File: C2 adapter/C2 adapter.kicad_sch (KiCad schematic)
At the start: 13 parts, among them J1 Conn_01x08_Pin, J2 Conn_02x05_Counter_Clockwise, J3 Conn_01x08_Socket, Q1 Q_NPN_BCE, U1 BAV23CLT1G

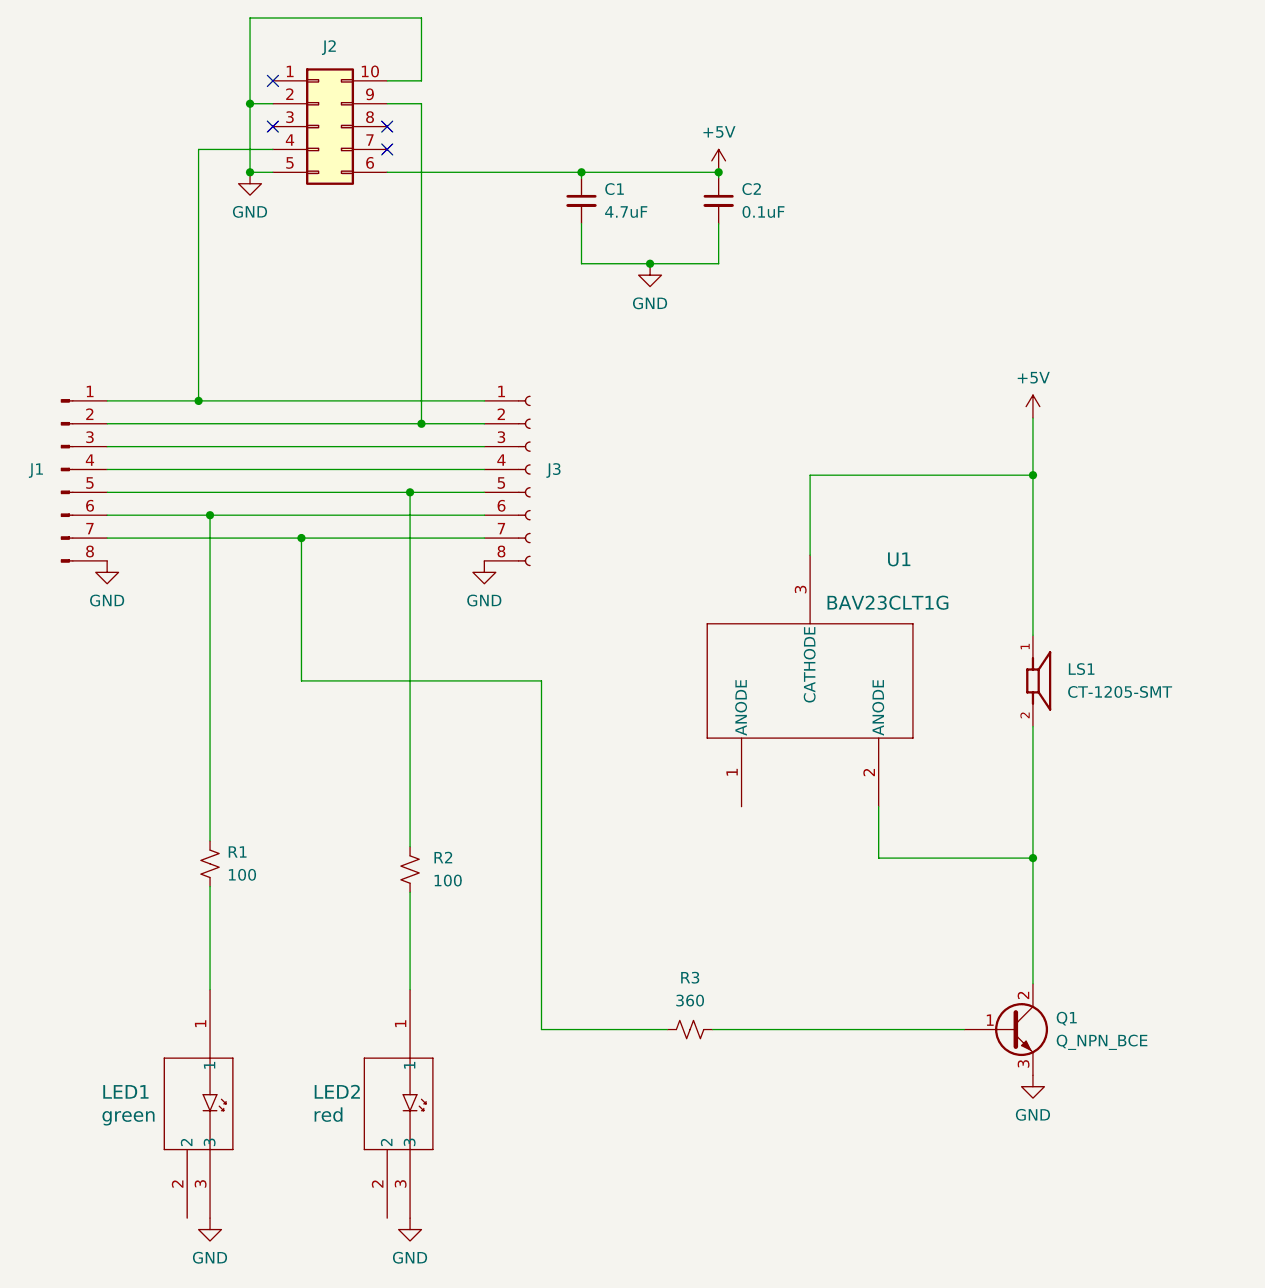
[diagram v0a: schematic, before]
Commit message: Add files via upload
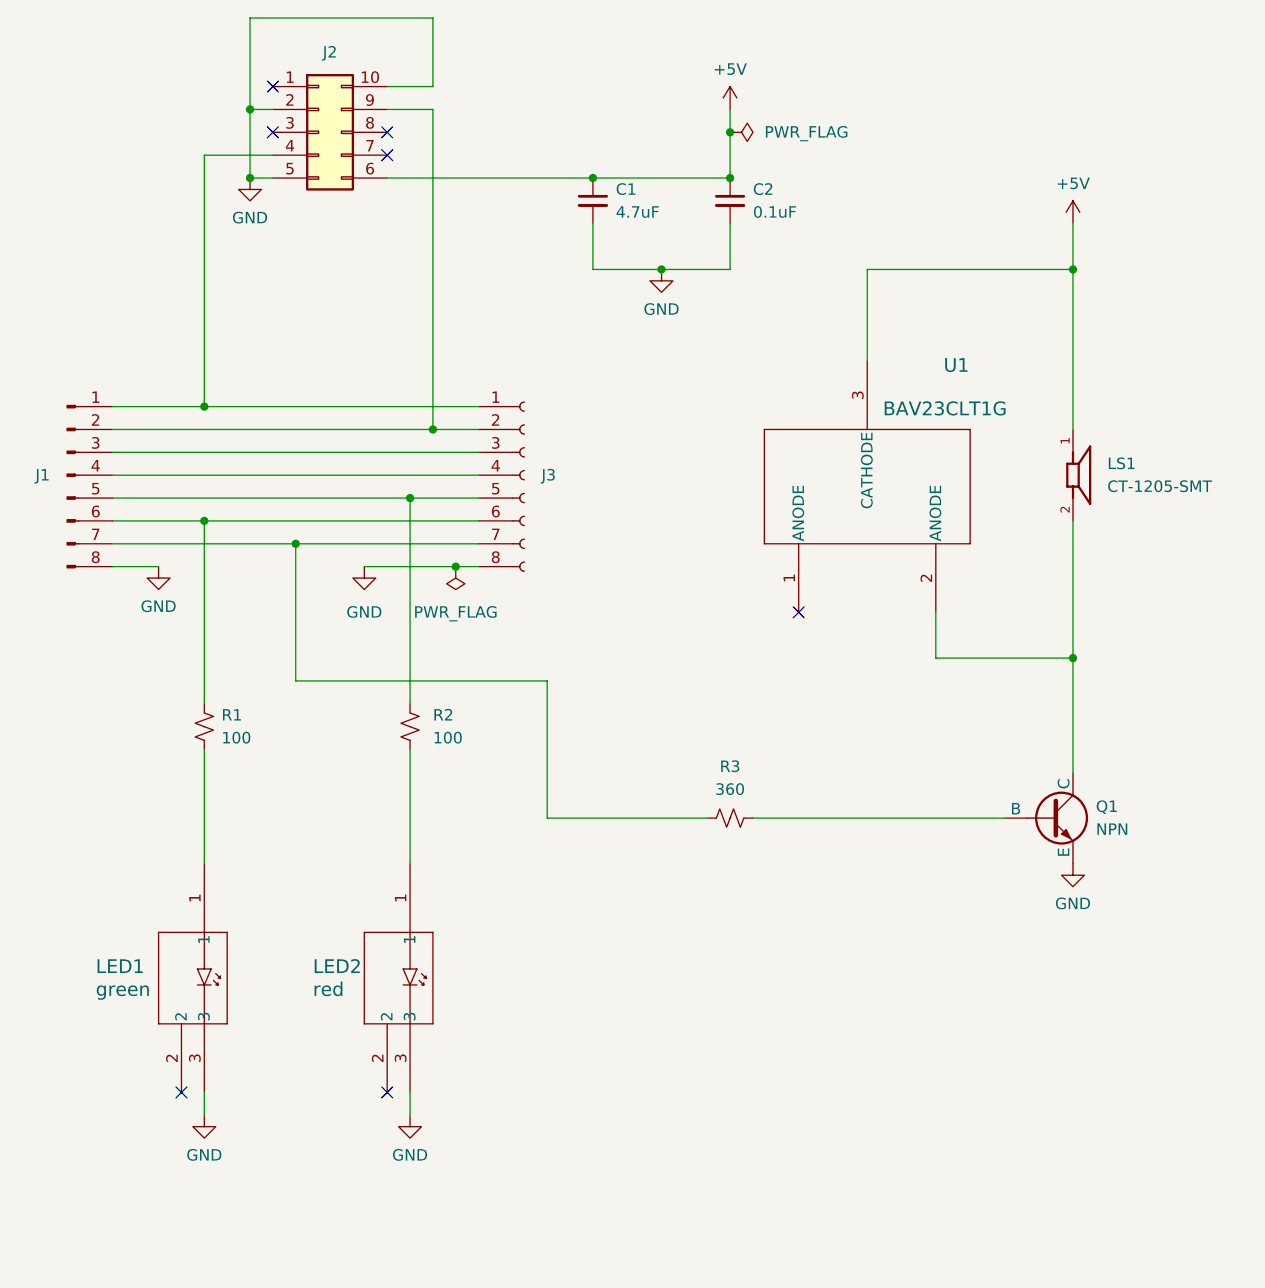
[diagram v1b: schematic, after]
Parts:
- removed Q1: Q_NPN_BCE, symbol Device:Q_NPN_BCE
- added Q1: NPN, NPN_Transitor:SOT95P240X110-3N, symbol Simulation_SPICE:NPN
- C1, C2: footprint (none) -> Capacitor_Tantalum_SMD:CP_EIA-1608-08_AVX-J_Pad1.25x1.05mm_HandSolder
- J1: footprint (none) -> Connector_PinHeader_2.00mm:PinHeader_1x08_P2.00mm_Horizontal
- J2: footprint (none) -> Connector_PinSocket_2.00mm:PinSocket_2x05_P2.00mm_Vertical
- J3: footprint (none) -> Connector_PinSocket_2.00mm:PinSocket_1x08_P2.00mm_Horizontal
- LED1: footprint SOT-23 -> LED Green:SOT-23
- LED2: footprint SOT-23 -> LED Red:SOT95P237X112-3N
- LS1: footprint CT-1205-SMT:CUI_CT-1205-SMT -> Buzzer_CT_1205_SMT_TR:CUI_CT-1205-SMT
- R1, R2, R3: footprint (none) -> Resistor_SMD:R_0201_0603Metric_Pad0.64x0.40mm_HandSolder
- U1: footprint SOT-23-3_1P4X3P040_ONS -> Diode array:SOT-23-3_1P4X3P040_ONS-L
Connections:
- net GND: now also Q1.3 (E)
- net at R3.2: now also Q1.2 (B)
- net at LS1.2, U1.2 (ANODE): now also Q1.1 (C)
- no-connect marks 4 -> 7
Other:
- moved on the sheet: C1, C2, J1, J2, J3, LED1, LED2, LS1, R1, R2, R3, U1
